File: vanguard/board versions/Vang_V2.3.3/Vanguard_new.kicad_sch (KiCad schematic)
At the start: 103 parts, among them J1 USB_C_Receptacle_USB2.0_16P, J2 Micro_SD_Card_Det1, J3 Conn_02x03_Odd_Even, J4 Conn_01x03, J5 Conn_01x03, J6 Conn_01x03, J7 Conn_01x02_Pin, Q1 BSS138, Q2 BSS138, Q3 BSS138, Q4 BSS138, U1 TXB0104D, U11 TPS82130SILR, U12 AP2112K-3.3, U3 ATSAMD11D14A-M, U4 BMP390L, U5 BD1020HFV-TR, U6 AT25DF641A-SH-T, U7 ATmega4809-A, U8 BNO055, U9 TPS61092, Y1 Crystal

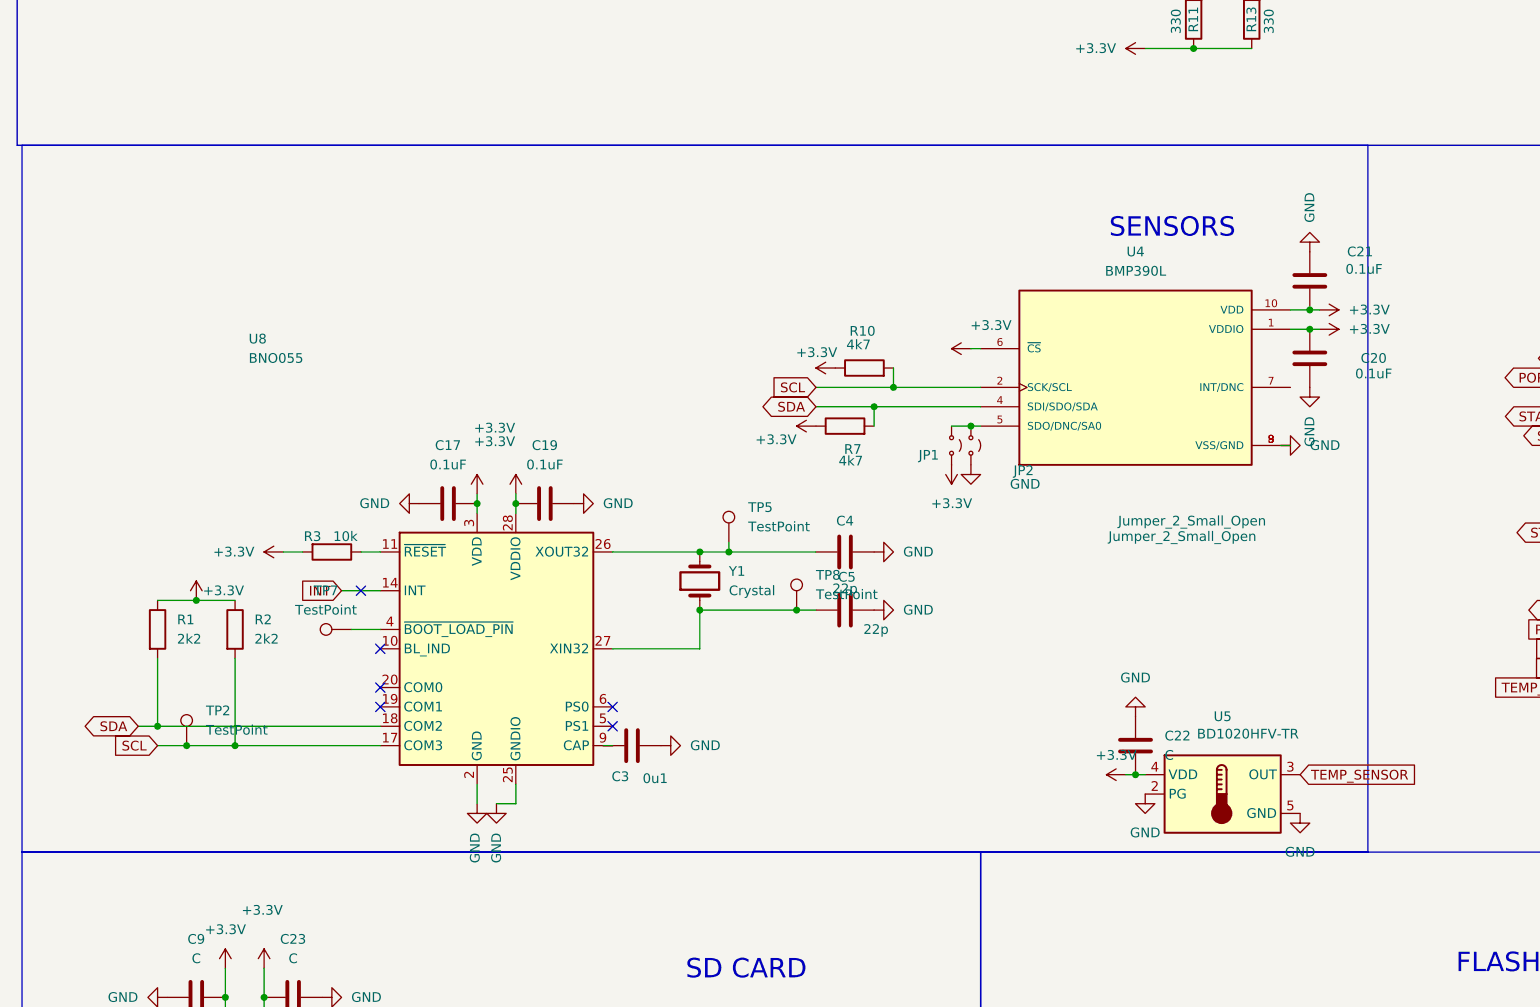
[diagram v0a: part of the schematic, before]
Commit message: 2.3.3 fix
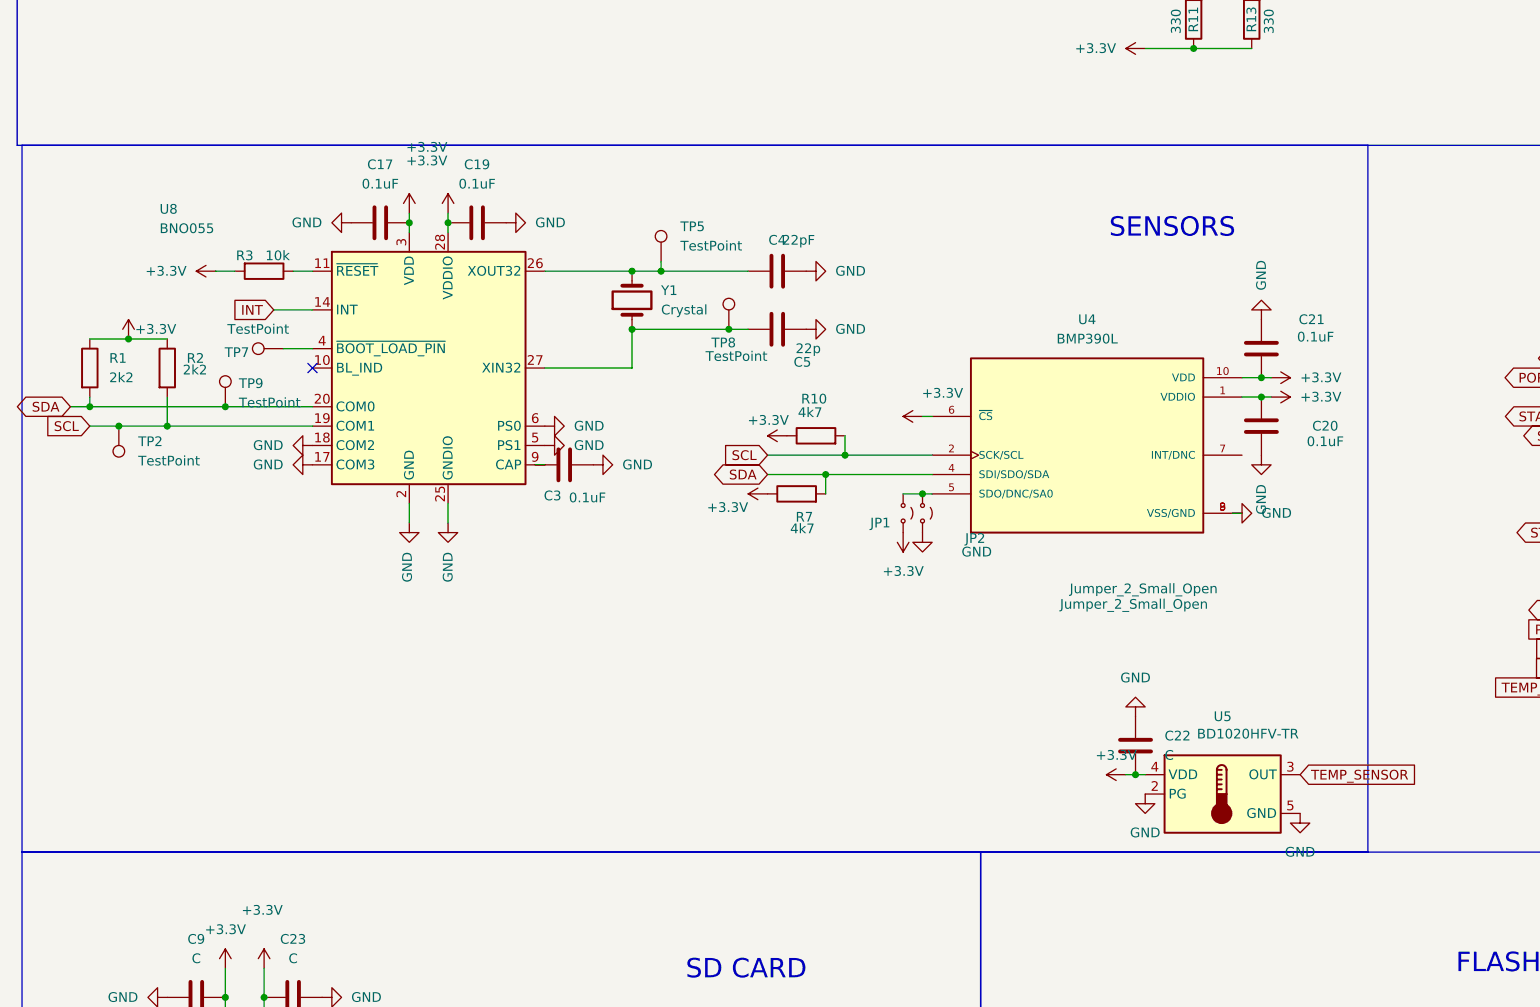
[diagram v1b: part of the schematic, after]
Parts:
- added TP9: TestPoint, TestPoint:TestPoint_Pad_1.0x1.0mm, symbol Connector:TestPoint
- C10, C11, C16, C17, C19, C20, C21, C22, C23, C6, C7, C9: footprint (none) -> Capacitor_SMD:C_0201_0603Metric
- C3: value 0u1 -> 0.1uF
- C4: value 22p -> 22pF
- R27, R28, R29, R30, R31, R35, R37, R38: footprint (none) -> Resistor_SMD:R_0402_1005Metric
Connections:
- net GND: now also U8.17 (COM3), U8.18 (COM2), U8.5 (PS1), U8.6 (PS0)
- net SCL: now also U8.19 (COM1); no longer U8.17 (COM3)
- net SDA: now also U8.20 (COM0), TP9.1; no longer U8.18 (COM2)
- no-connect marks 38 -> 33
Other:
- moved on the sheet: C17, C19, C20, C21, C3, C4, C5, JP1, JP2, R1, R10, R2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
